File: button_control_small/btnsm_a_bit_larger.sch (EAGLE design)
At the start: 23 parts, among them IC1 TINY13V-10SSU, Q1 IRF8788

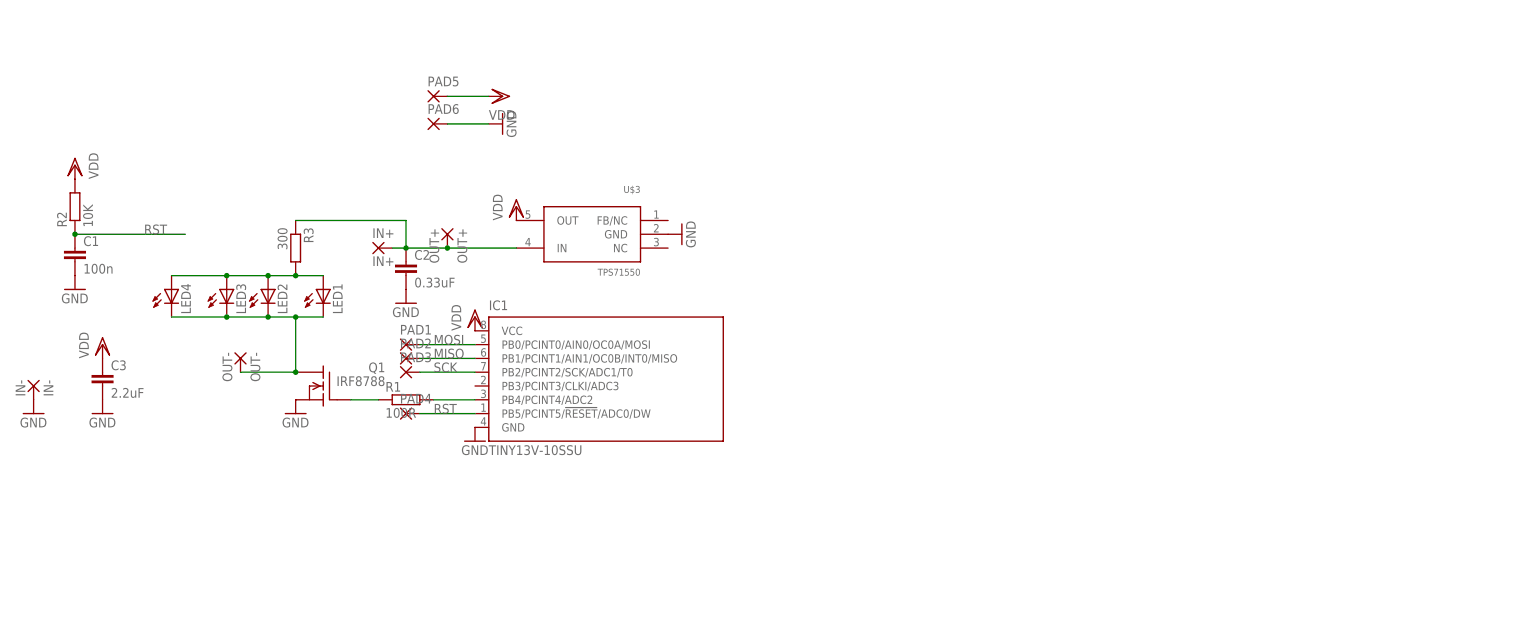
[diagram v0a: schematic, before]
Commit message: Add files via upload
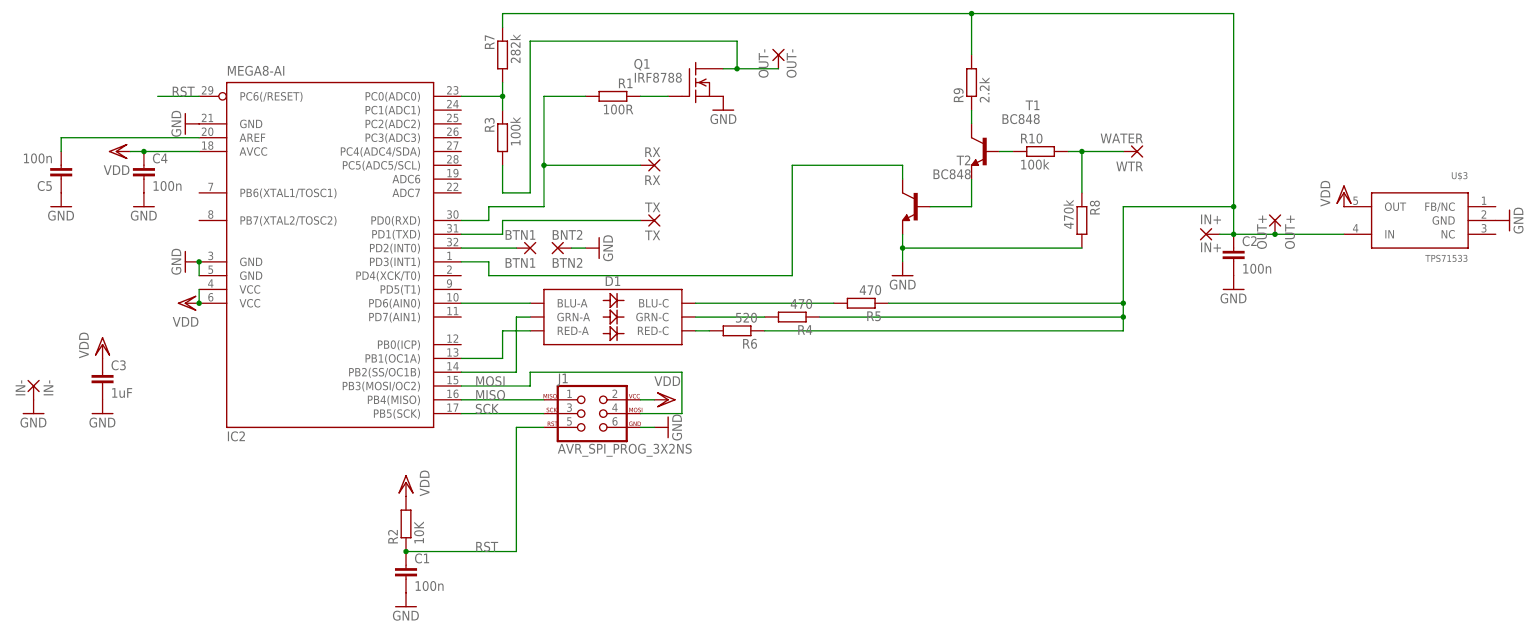
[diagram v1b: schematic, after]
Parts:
- removed IC1: TINY13V-10SSU, atmel:TINY13V-10SSU
- removed LED1, LED3: (no value), eagle-ltspice:LED_ESML0603
- removed LED2, LED4: (no value), led:LED5MM
- removed PAD1, PAD2, PAD3, PAD4, PAD5, PAD6: (no value), wirepad:1,6/0,9
- added BTN1: BTN1, wirepad:1,6/0,9
- added BTN2: BNT2, wirepad:1,6/0,9
- added C4, C5: 100n, resistor:C-EUC0603
- added D1: (no value), SparkFun-LED:LED-RGBNO_IC
- added IC2: MEGA8-AI, atmel:MEGA8-AI
- added J1: AVR_SPI_PROG_3X2NS, SparkFun-Connectors:AVR_SPI_PROG_3X2NS
- added R10: 100k, rcl:R-EU_R0402
- added R4, R5: 470, rcl:R-EU_R0402
- added R6: 520, rcl:R-EU_R0402
- added R7: 282k, rcl:R-EU_R0402
- added R8: 470k, rcl:R-EU_R0402
- added R9: 2.2k, rcl:R-EU_R0402
- added RX: RX, wirepad:1,6/0,9
- added T1, T2: BC848, transistor-neu-to92:BC848
- added TX: TX, wirepad:1,6/0,9
- added WTR: WATER, wirepad:1,6/0,9
- C2: value 0.33uF -> 100n
- C3: value 2.2uF -> 1uF; device resistor:C-EUC0603 -> resistor:C-EUC0805
- R3: value 300 -> 100k
- U$3: value TPS71550 -> TPS71533
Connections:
- removed net N$1: IC1.PB4/PCINT4/ADC2, R1.2
- removed net N$3: C2.1, IN+.P, OUT+.P, R3.1, U$3.IN
- new net ADC0: IC2.PC0(ADC0), R3.1, R7.2
- new net AREF: C5.2, IC2.AREF
- new net BTN1: BTN1.P, IC2.PD2(INT0)
- new net N$13: T1.E, T2.B
- new net N$16: R10.2, R8.1, WTR.P
- new net N$17: R10.1, T1.B
- new net N$18: R9.1, T1.C
- new net N$7: D1.GRN-C, R4.2
- new net N$8: D1.BLU-C, R5.2
- new net PWM0: D1.BLU-A, IC2.PD6(AIN0)
- new net PWM1: D1.GRN-A, IC2.PB2(SS/OC1B)
- new net PWM2: D1.RED-A, IC2.PB1(OC1A)
- new net RX: IC2.PD0(RXD), R1.2, RX.P
- new net TX: IC2.PD1(TXD), TX.P
- new net VIN: C2.1, IN+.P, OUT+.P, R4.1, R5.1, R6.1, R7.1, R9.2, U$3.IN
- new net WTR: IC2.PD3(INT1), T2.C
- net GND: now also BTN2.P, C4.2, C5.1, IC2.GND, IC2.GND@1, IC2.GND@2, J1.6, R8.2, T2.E; no longer IC1.GND, PAD6.P
- net MISO: now also IC2.PB4(MISO), J1.1; no longer IC1.PB1/PCINT1/AIN1/OC0B/INT0/MISO, PAD2.P
- net MOSI: now also IC2.PB3(MOSI/OC2), J1.4; no longer IC1.PB0/PCINT0/AIN0/OC0A/MOSI, PAD1.P
- net N$4: now also R3.2; no longer LED1.C, LED2.C, LED3.C, LED4.C
- net N$6: now also D1.RED-C, R6.2; no longer LED1.A, LED2.A, LED3.A, LED4.A, R3.2
- net RST: now also IC2.PC6(/RESET), J1.5; no longer IC1.PB5/PCINT5/!RESET!/ADC0/DW, PAD4.P
- net SCK: now also IC2.PB5(SCK), J1.3; no longer IC1.PB2/PCINT2/SCK/ADC1/T0, PAD3.P
- net VDD: now also C4.1, IC2.AVCC, IC2.VCC@1, IC2.VCC@2, J1.2; no longer IC1.VCC, PAD5.P
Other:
- moved on the sheet: C1, C2, IN+, OUT+, OUT-, Q1, R1, R2, R3, U$3
